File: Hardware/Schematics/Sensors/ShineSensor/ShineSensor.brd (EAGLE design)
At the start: 12.7 x 19.1 mm, 6 parts, among them IC1 DS18B20, Q1 BSS138

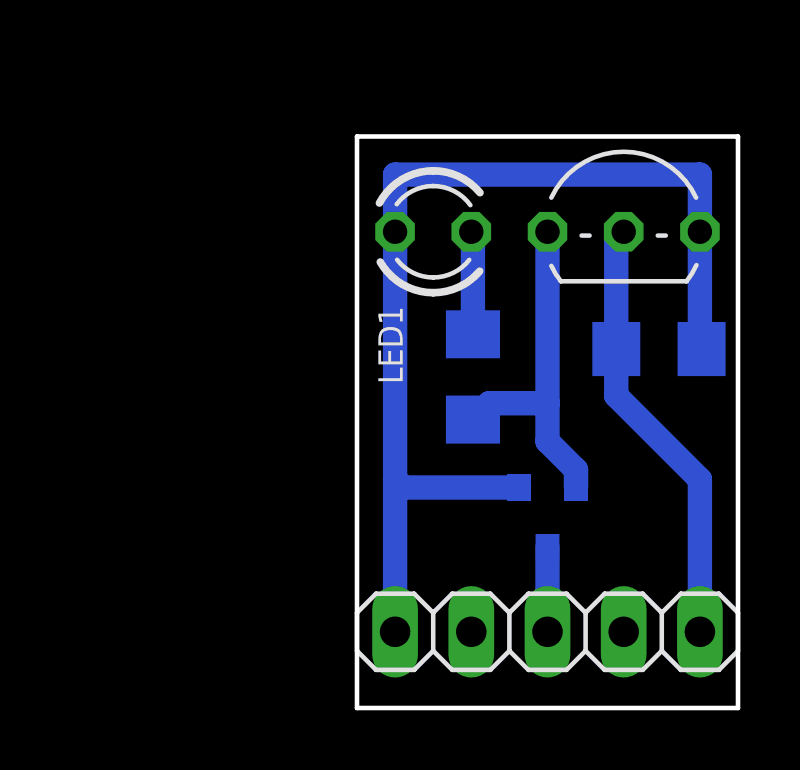
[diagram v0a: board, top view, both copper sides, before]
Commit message: commit
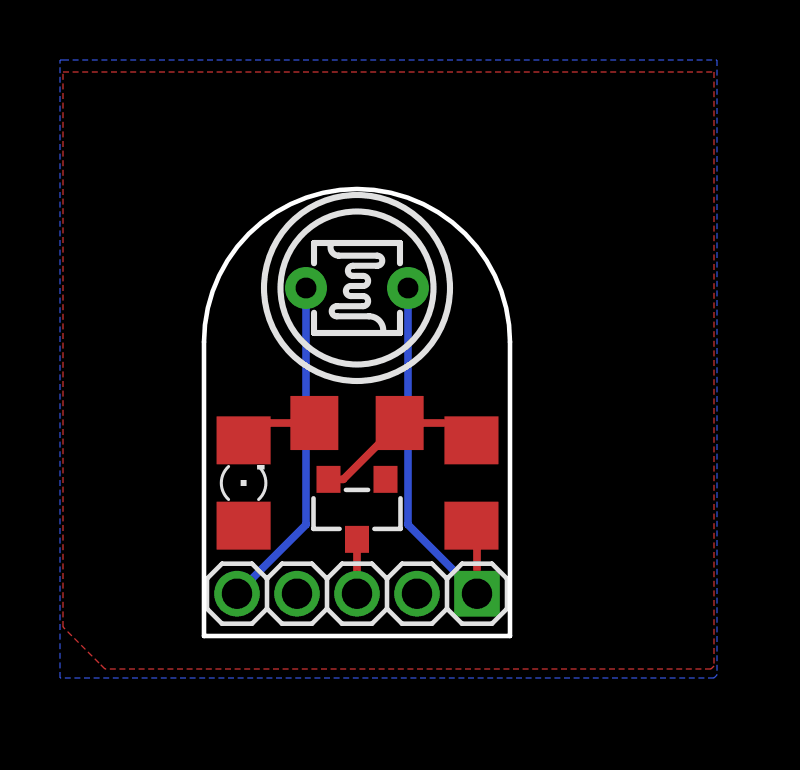
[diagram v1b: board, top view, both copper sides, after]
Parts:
- removed IC1: DS18B20, 1wire:TO92-
- removed LED1: 3mm 2ma, led:LED3MM
- added LED2: (no value), led:1206
- added PH1: A10, photo-elements:T0-46-A10XX
- JP1: device pinhead:1X05 -> pinhead:1_05X2MM
- R1: value 1k -> 330
- R2: value 330 -> 1k
- moved R1 7.68 mm to (3.81, 7.50), flipped to the top, turned to 90 degrees
- moved JP1 6.48 mm to (0.00, 3.81)
- moved Q1 6.36 mm to (0.00, 6.62), flipped to the top
- moved R2 4.16 mm to (0.00, 9.50), flipped to the top, turned to 180 degrees
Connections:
- removed net N$1: IC1.3, JP1.5, LED1.A, Q1.1, R1.1
- removed net N$4: IC1.1, Q1.2, R2.1
- removed net N$5: IC1.2, JP1.1, R1.2
- new net 3V3: JP1.5, LED2.A, PH1.2, Q1.1
- new net N$13: JP1.1, PH1.1, R1.1
- new net N$14: Q1.2, R1.2, R2.1
- net N$2: now also LED2.C; no longer LED1.K
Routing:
- net N$1: track 35.5 -> 0.00 mm
- net N$5: track 14.6 -> 0.00 mm
- net N$13: track 0.00 -> 13.5 mm
- net N$4: track 11.6 -> 0.00 mm
- net 3V3: track 0.00 -> 11.1 mm
- net N$14: track 0.00 -> 5.78 mm
- net N$3: track 2.81 -> 1.81 mm
- net N$2: track 3.44 -> 2.60 mm
- added copper zone on layer 1, net 3V3
- added copper zone on layer 16, net GND
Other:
- board size 12.7 x 19.1 mm -> 10.2 x 14.9 mm
- board text added: "JLCPCB"
- board text added: "Sponsored"
- board text added: "by"
